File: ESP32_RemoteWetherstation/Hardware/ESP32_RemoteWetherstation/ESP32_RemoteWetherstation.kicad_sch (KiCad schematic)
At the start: 5 parts, among them J301 BOOT, J302 UART, U303 ESP32-S3-MINI-1

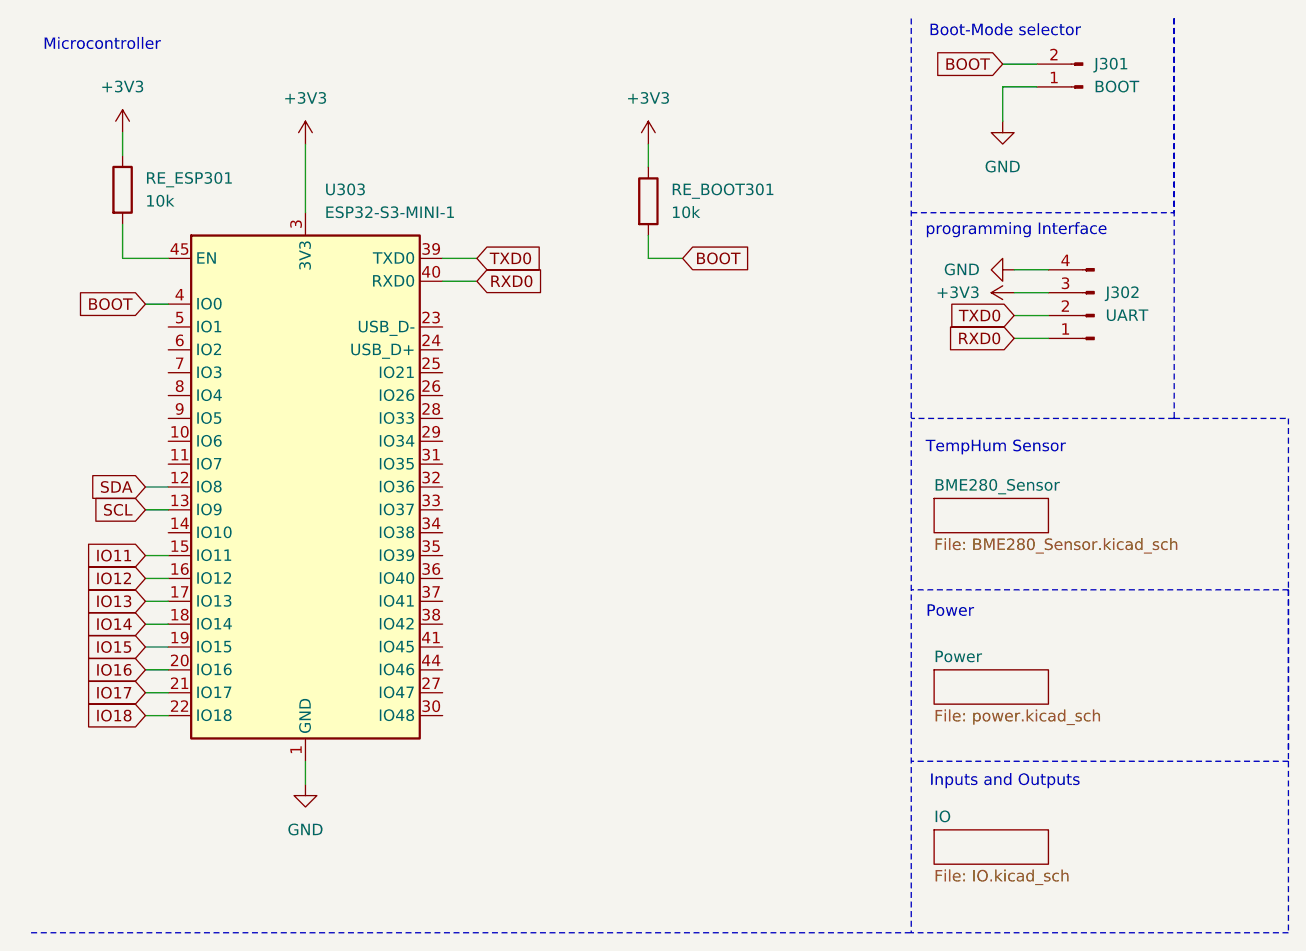
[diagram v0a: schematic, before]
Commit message: placed all comps onesided (#11)
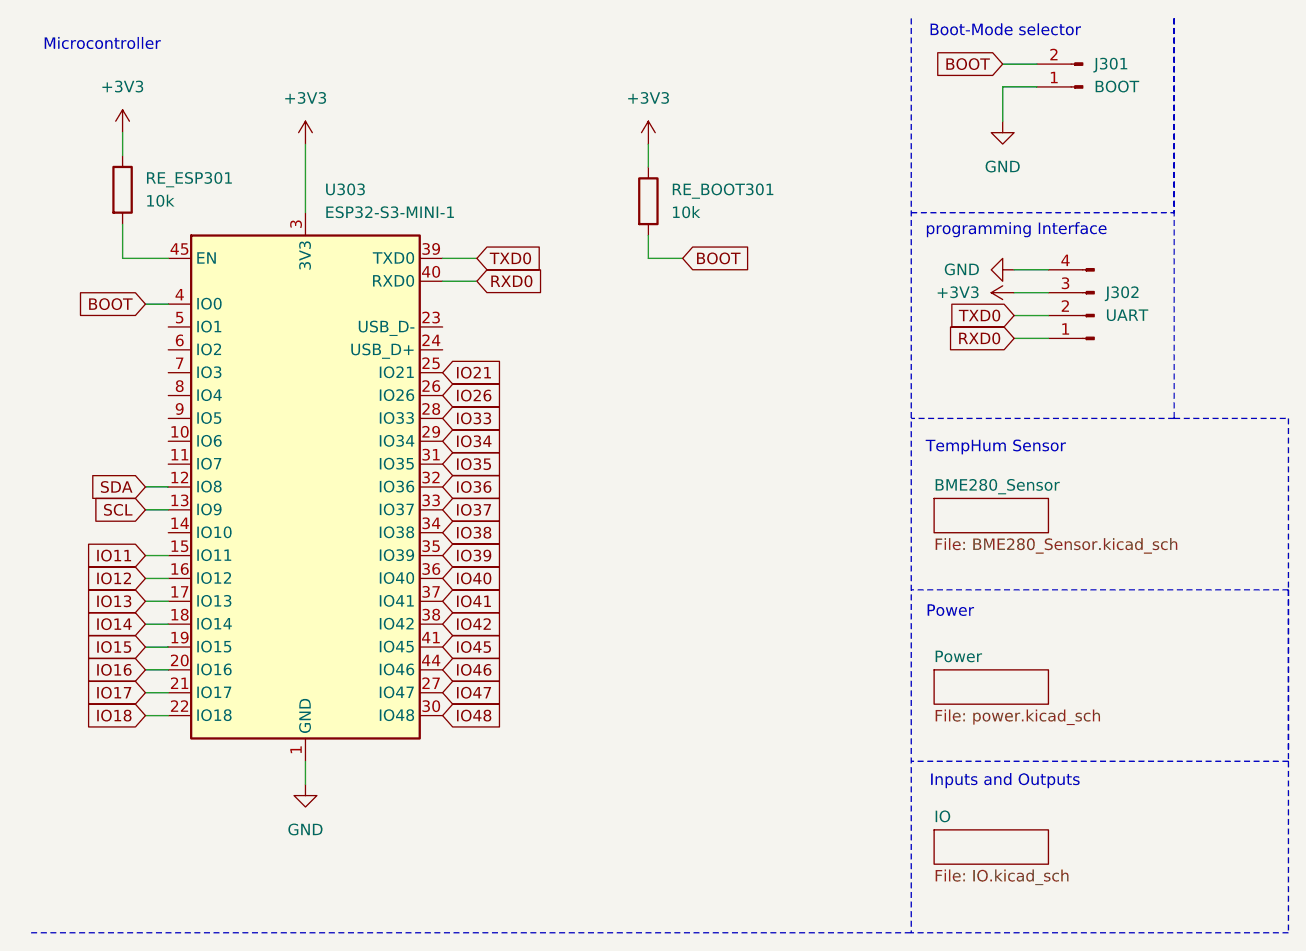
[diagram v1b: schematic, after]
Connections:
- net IO21: now reaches U303.25 (IO21)
- net IO26: now reaches U303.26 (IO26)
- net IO47: now reaches U303.27 (IO47)
- net IO33: now reaches U303.28 (IO33)
- net IO34: now reaches U303.29 (IO34)
- net IO48: now reaches U303.30 (IO48)
- net IO35: now reaches U303.31 (IO35)
- net IO36: now reaches U303.32 (IO36)
- net IO37: now reaches U303.33 (IO37)
- net IO38: now reaches U303.34 (IO38)
- net IO39: now reaches U303.35 (IO39)
- net IO40: now reaches U303.36 (IO40)
- net IO41: now reaches U303.37 (IO41)
- net IO42: now reaches U303.38 (IO42)
- net IO45: now reaches U303.41 (IO45)
- net IO46: now reaches U303.44 (IO46)
